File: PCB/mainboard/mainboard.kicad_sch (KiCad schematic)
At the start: 44 parts, among them J1 TO_BATT, J2 TO_LED, J3 FAN, Q1 Q_NPN_BCE, Q2 Q_NMOS_DGS, Q3 Q_NMOS_DGS, U1 AP63203WU, U2 ZXLD1370, U3 AP63205WU

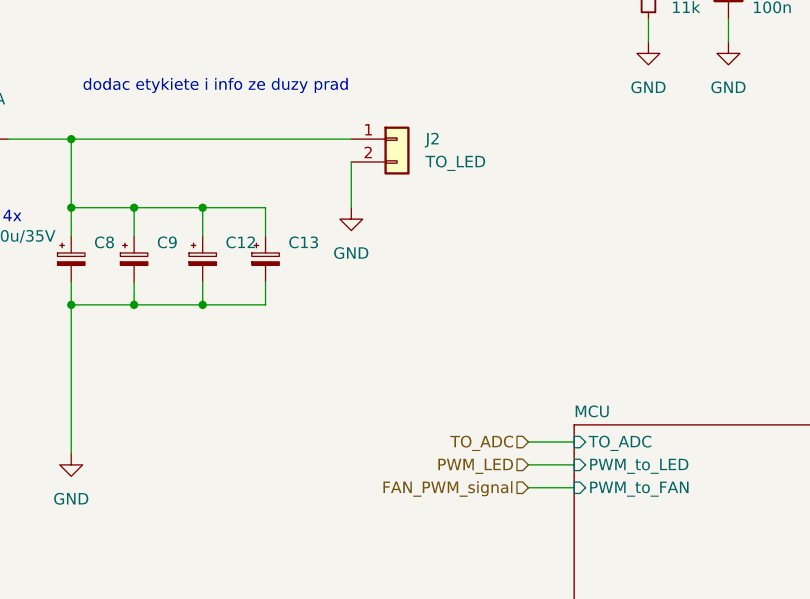
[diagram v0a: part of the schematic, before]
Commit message: small details and sugestions
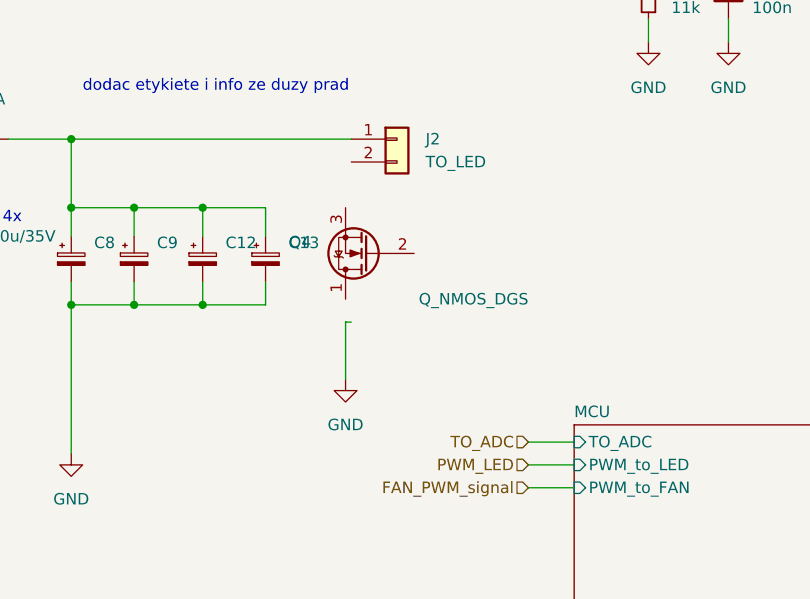
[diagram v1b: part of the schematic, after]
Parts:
- added Q4: Q_NMOS_DGS, symbol Device:Q_NMOS_DGS
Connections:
- net GND: no longer J2.2 (Pin_2)
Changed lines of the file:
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@@
     (stroke (width 0) (type default))
   )
-  (wire (pts (xy 159.385 55.88) (xy 159.385 60.96))
+  (wire (pts (xy 158.75 73.66) (xy 158.75 80.01))
     (stroke (width 0) (type default))
   )
@@
   )
   (wire (pts (xy 262.255 60.325) (xy 262.255 61.595))
+    (stroke (width 0) (type default))
+  )
+  (wire (pts (xy 158.75 73.66) (xy 159.385 73.66))
     (stroke (width 0) (type default))
   )
@@
     )
   )
-  (symbol (lib_id "power:GND") (at 159.385 60.96 0) (unit 1)
-    (in_bom yes) (on_board yes) (dnp no) (fields_autoplaced)
-    (property "Reference" "#PWR017" (at 159.385 67.31 0)
-      (effects (font (size 1.27 1.27)) hide)
-    )
-    (property "Value" "GND" (at 159.385 66.04 0)
-      (effects (font (size 1.27 1.27)))
-    )
-    (property "Footprint" "" (at 159.385 60.96 0)
-      (effects (font (size 1.27 1.27)) hide)
-    )
-    (property "Datasheet" "" (at 159.385 60.96 0)
+  (symbol (lib_id "power:GND") (at 158.75 80.01 0) (unit 1)
+    (in_bom yes) (on_board yes) (dnp no) (fields_autoplaced)
+    (property "Reference" "#PWR017" (at 158.75 86.36 0)
+      (effects (font (size 1.27 1.27)) hide)
+    )
+    (property "Value" "GND" (at 158.75 85.09 0)
+      (effects (font (size 1.27 1.27)))
+    )
+    (property "Footprint" "" (at 158.75 80.01 0)
+      (effects (font (size 1.27 1.27)) hide)
+    )
+    (property "Datasheet" "" (at 158.75 80.01 0)
       (effects (font (size 1.27 1.27)) hide)
     )
@@
         )
       )
+    )
+  )
+  (symbol (lib_id "Device:Q_NMOS_DGS") (at 161.29 66.04 180) (unit 1)
+    (in_bom yes) (on_board yes) (dnp no)
+    (property "Reference" "Q4" (at 154.94 64.77 0)
+      (effects (font (size 1.27 1.27)) (justify left))
+    )
+    (property "Value" "Q_NMOS_DGS" (at 179.07 71.12 0)
+      (effects (font (size 1.27 1.27)) (justify left))
+    )
+    (property "Footprint" "" (at 156.21 68.58 0)
+      (effects (font (size 1.27 1.27)) hide)
+    )
+    (property "Datasheet" "~" (at 161.29 66.04 0)
+      (effects (font (size 1.27 1.27)) hide)
+    )
+    (pin "1")
+    (pin "2")
+    (pin "3")
+    (instances
+      (project "mainboard"
+        (path "/e63e39d7-6ac0-4ffd-8aa3-1841a4541b55"
+          (reference "Q4") (unit 1)
+        )
+      )
